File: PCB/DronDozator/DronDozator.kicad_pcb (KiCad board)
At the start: 2 copper layers, 7 parts, among them U1 LM2596

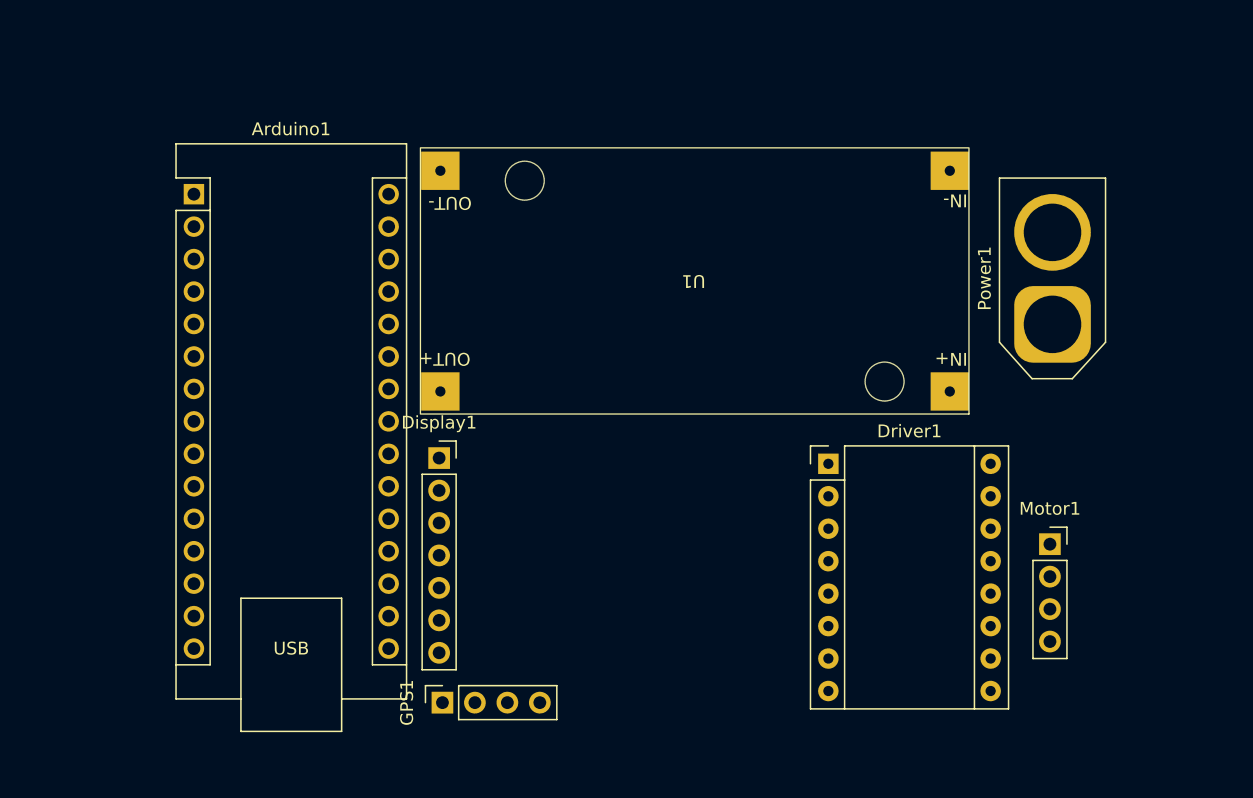
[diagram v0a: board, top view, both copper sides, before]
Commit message: Finalized schem
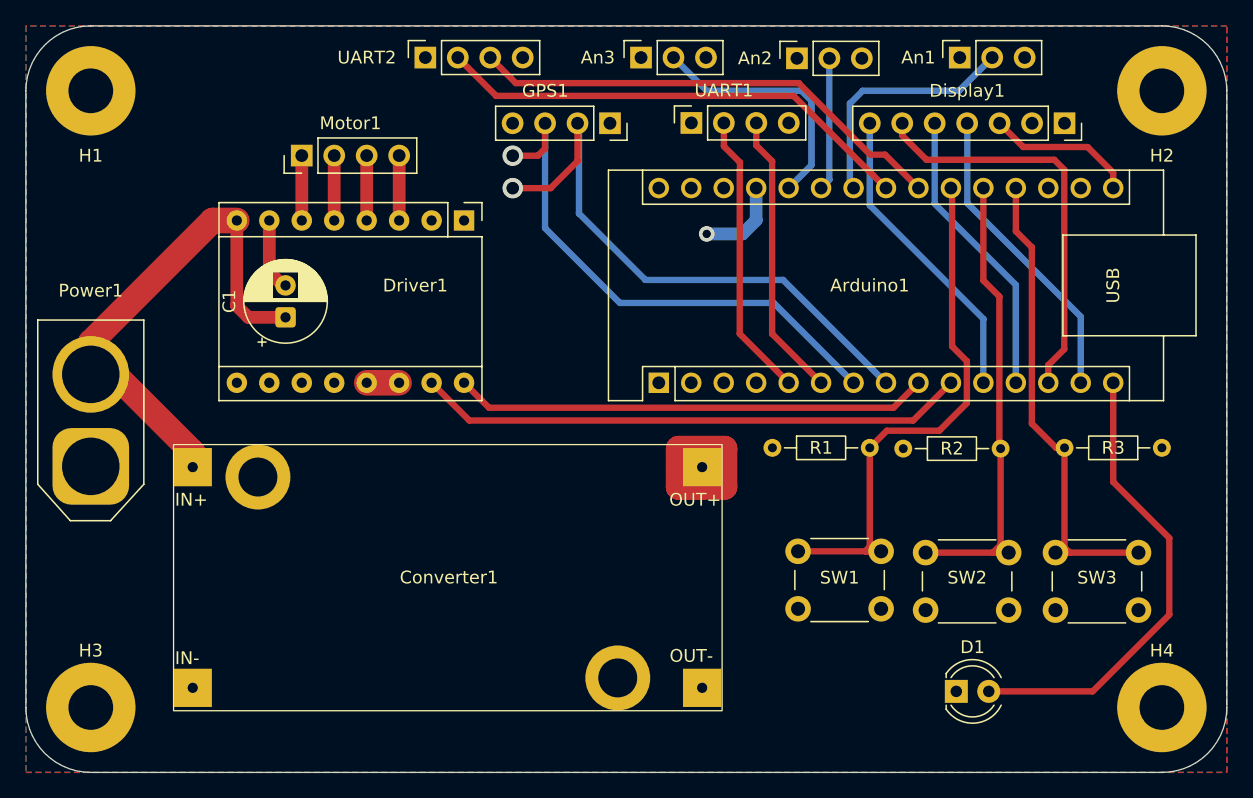
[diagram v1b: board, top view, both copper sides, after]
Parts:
- added An1: Conn_01x03_Socket, Connector_PinSocket_2.54mm:PinSocket_1x03_P2.54mm_Vertical, F.Cu at (95.9, 17.7)
- added An2: Conn_01x03_Socket, Connector_PinSocket_2.54mm:PinSocket_1x03_P2.54mm_Vertical, F.Cu at (83.2, 17.8)
- added An3: Conn_01x03_Socket, Connector_PinSocket_2.54mm:PinSocket_1x03_P2.54mm_Vertical, F.Cu at (71.0, 17.7)
- added C1: 100uF, Capacitor_THT:CP_Radial_D6.3mm_P2.50mm, F.Cu at (43.2, 38.0)
- added D1: LED, LED_THT:LED_D4.0mm, F.Cu at (95.7, 67.3)
- added H1: MountingHole_Pad, MountingHole:MountingHole_3.5mm_Pad, F.Cu at (27.9, 20.3)
- added H2: MountingHole_Pad, MountingHole:MountingHole_3.5mm_Pad, F.Cu at (111.8, 20.3)
- added H3: MountingHole_Pad, MountingHole:MountingHole_3.5mm_Pad, F.Cu at (27.9, 68.6)
- added H4: MountingHole_Pad, MountingHole:MountingHole_3.5mm_Pad, F.Cu at (111.8, 68.6)
- added R1: 10k, Resistor_THT:R_Axial_DIN0204_L3.6mm_D1.6mm_P7.62mm_Horizontal, F.Cu at (81.3, 48.3)
- added R2: 10k, Resistor_THT:R_Axial_DIN0204_L3.6mm_D1.6mm_P7.62mm_Horizontal, F.Cu at (91.5, 48.3)
- added R3: 10k, Resistor_THT:R_Axial_DIN0204_L3.6mm_D1.6mm_P7.62mm_Horizontal, F.Cu at (111.8, 48.3)
- added SW1: SW_Push, Button_Switch_THT:SW_PUSH_6mm, F.Cu at (83.3, 56.4)
- added SW2: SW_Push, Button_Switch_THT:SW_PUSH_6mm, F.Cu at (93.3, 56.5)
- added SW3: SW_Push, Button_Switch_THT:SW_PUSH_6mm, F.Cu at (103.4, 56.5)
- added UART1: Conn_01x04_Socket, Connector_PinSocket_2.54mm:PinSocket_1x04_P2.54mm_Vertical, F.Cu at (74.9, 22.8)
- added UART2: Conn_01x04_Socket, Connector_PinSocket_2.54mm:PinSocket_1x04_P2.54mm_Vertical, F.Cu at (54.1, 17.7)
- Motor1: footprint Connector_PinSocket_2.54mm:PinSocket_1x04_P2.54mm_Vertical -> Connector_PinHeader_2.54mm:PinHeader_1x04_P2.54mm_Vertical
- moved Power1 76.1 mm to (27.9, 49.7)
- moved Motor1 66.0 mm to (44.5, 25.4), turned to 90 degrees
- moved Converter1 62.3 mm to (34.4, 48.0), turned to 0 degrees
- moved Display1 55.5 mm to (104.1, 22.9), turned to -90 degrees
- moved GPS1 47.2 mm to (68.6, 22.9), turned to -90 degrees
- moved Arduino1 39.3 mm to (72.4, 43.2), turned to 90 degrees
- moved Driver1 34.3 mm to (57.1, 30.5), turned to -90 degrees
- renumbered U1 to Converter1
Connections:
- Arduino1 pad 10: unconnected-(Arduino1-D7-Pad10) -> /STEP
- Arduino1 pad 11: unconnected-(Arduino1-D8-Pad11) -> /CS
- Arduino1 pad 12: unconnected-(Arduino1-D9-Pad12) -> /RES
- Arduino1 pad 13: unconnected-(Arduino1-D10-Pad13) -> /DC
- Arduino1 pad 14: unconnected-(Arduino1-D11-Pad14) -> /MOSI
- Arduino1 pad 15: unconnected-(Arduino1-D12-Pad15) -> /LED
- Arduino1 pad 16: unconnected-(Arduino1-D13-Pad16) -> /CLK
- Arduino1 pad 19: unconnected-(Arduino1-A0-Pad19) -> /SW3
- Arduino1 pad 20: unconnected-(Arduino1-A1-Pad20) -> /SW2
- Arduino1 pad 21: unconnected-(Arduino1-A2-Pad21) -> /SW1
- Arduino1 pad 22: unconnected-(Arduino1-A3-Pad22) -> /UART2_TX
- Arduino1 pad 23: unconnected-(Arduino1-A4-Pad23) -> /UART2_RX
- Arduino1 pad 24: unconnected-(Arduino1-A5-Pad24) -> /Analog1
- Arduino1 pad 25: unconnected-(Arduino1-A6-Pad25) -> /Analog2
- Arduino1 pad 26: unconnected-(Arduino1-A7-Pad26) -> /Analog3
- Arduino1 pad 27: unconnected-(Arduino1-+5V-Pad27) -> +5V
- Arduino1 pad 29: unconnected-(Arduino1-GND-Pad29) -> GND
- Arduino1 pad 4: unconnected-(Arduino1-GND-Pad4) -> GND
- Arduino1 pad 5: unconnected-(Arduino1-D2-Pad5) -> /UART1_RX
- Arduino1 pad 6: unconnected-(Arduino1-D3-Pad6) -> /UART1_TX
- Arduino1 pad 7: unconnected-(Arduino1-D4-Pad7) -> /ARD_RX
- Arduino1 pad 8: unconnected-(Arduino1-D5-Pad8) -> /ARD_TX
- Arduino1 pad 9: unconnected-(Arduino1-D6-Pad9) -> /DIR
- Converter1 pad 1: unconnected-(U1-IN+-Pad1) -> VCC
- Converter1 pad 2: unconnected-(U1-IN--Pad2) -> GND
- Converter1 pad 3: unconnected-(U1-OUT+-Pad3) -> +5V
- Converter1 pad 4: unconnected-(U1-OUT--Pad4) -> GND
- Display1 pad 1: unconnected-(Display1-Pin_1-Pad1) -> GND
- Display1 pad 2: unconnected-(Display1-Pin_2-Pad2) -> +5V
- Display1 pad 3: unconnected-(Display1-Pin_3-Pad3) -> /CLK
- Display1 pad 4: unconnected-(Display1-Pin_4-Pad4) -> /MOSI
- Display1 pad 5: unconnected-(Display1-Pin_5-Pad5) -> /RES
- Display1 pad 6: unconnected-(Display1-Pin_6-Pad6) -> /DC
- Display1 pad 7: unconnected-(Display1-Pin_7-Pad7) -> /CS
- Driver1 pad 1: unconnected-(Driver1-GND-Pad1) -> GND
- Driver1 pad 10: unconnected-(Driver1-MS1-Pad10) -> GND
- Driver1 pad 11: unconnected-(Driver1-MS2-Pad11) -> +5V
- Driver1 pad 12: unconnected-(Driver1-MS3-Pad12) -> GND
- Driver1 pad 13: unconnected-(Driver1-~{RESET}-Pad13) -> Net-(Driver1-~{RESET})
- Driver1 pad 14: unconnected-(Driver1-~{SLEEP}-Pad14) -> Net-(Driver1-~{RESET})
- Driver1 pad 15: unconnected-(Driver1-STEP-Pad15) -> /STEP
- Driver1 pad 16: unconnected-(Driver1-DIR-Pad16) -> /DIR
- Driver1 pad 2: unconnected-(Driver1-VDD-Pad2) -> +5V
- Driver1 pad 3: unconnected-(Driver1-1B-Pad3) -> Net-(Driver1-1B)
- Driver1 pad 4: unconnected-(Driver1-1A-Pad4) -> Net-(Driver1-1A)
- Driver1 pad 5: unconnected-(Driver1-2A-Pad5) -> Net-(Driver1-2A)
- Driver1 pad 6: unconnected-(Driver1-2B-Pad6) -> Net-(Driver1-2B)
- Driver1 pad 7: unconnected-(Driver1-GND-Pad7) -> GND
- Driver1 pad 8: unconnected-(Driver1-VMOT-Pad8) -> VCC
- Driver1 pad 9: unconnected-(Driver1-~{ENABLE}-Pad9) -> GND
- GPS1 pad 1: unconnected-(GPS1-Pin_1-Pad1) -> +5V
- GPS1 pad 2: unconnected-(GPS1-Pin_2-Pad2) -> /ARD_TX
- GPS1 pad 3: unconnected-(GPS1-Pin_3-Pad3) -> /ARD_RX
- GPS1 pad 4: unconnected-(GPS1-Pin_4-Pad4) -> GND
- Motor1 pad 1: unconnected-(Motor1-Pin_1-Pad1) -> Net-(Driver1-2B)
- Motor1 pad 2: unconnected-(Motor1-Pin_2-Pad2) -> Net-(Driver1-2A)
- Motor1 pad 3: unconnected-(Motor1-Pin_3-Pad3) -> Net-(Driver1-1A)
- Motor1 pad 4: unconnected-(Motor1-Pin_4-Pad4) -> Net-(Driver1-1B)
- Power1 pad 1: unconnected-(Power1-Pin_1-Pad1) -> GND
- Power1 pad 2: unconnected-(Power1-Pin_2-Pad2) -> VCC
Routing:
- net /ARD_TX: track 0.00 -> 45.5 mm, vias 0 -> 1
- net /STEP: track 0.00 -> 43.1 mm
- net /SW1: track 0.00 -> 42.4 mm
- net /ARD_RX: track 0.00 -> 42.1 mm, vias 0 -> 1
- net VCC: track 0.00 -> 40.4 mm
- net /UART2_RX: track 0.00 -> 37.7 mm
- net /UART2_TX: track 0.00 -> 37.7 mm
- net /DIR: track 0.00 -> 37.2 mm
- net /SW3: track 0.00 -> 37.2 mm
- net /SW2: track 0.00 -> 37.1 mm
- net /LED: track 0.00 -> 36.6 mm
- net /DC: track 0.00 -> 31.9 mm
- net /MOSI: track 0.00 -> 24.0 mm
- net /CS: track 0.00 -> 24.0 mm
- net +5V: track 0.00 -> 23.4 mm, vias 0 -> 1
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- added copper zone on F.Cu, net +5V
- added copper zone on B.Cu, net GND
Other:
- board outline added: 94 x 58.4 mm
